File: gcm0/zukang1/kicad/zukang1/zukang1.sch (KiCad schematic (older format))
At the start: 26 parts, among them J1 Conn_01x02_Male, U1 L7805, U2 LM1117-3.3, U3 74HC595, U4 STM32F030F4Px, U5 Si5351A-B-GT, Y1 Crystal, Y2 Crystal_GND24_Small

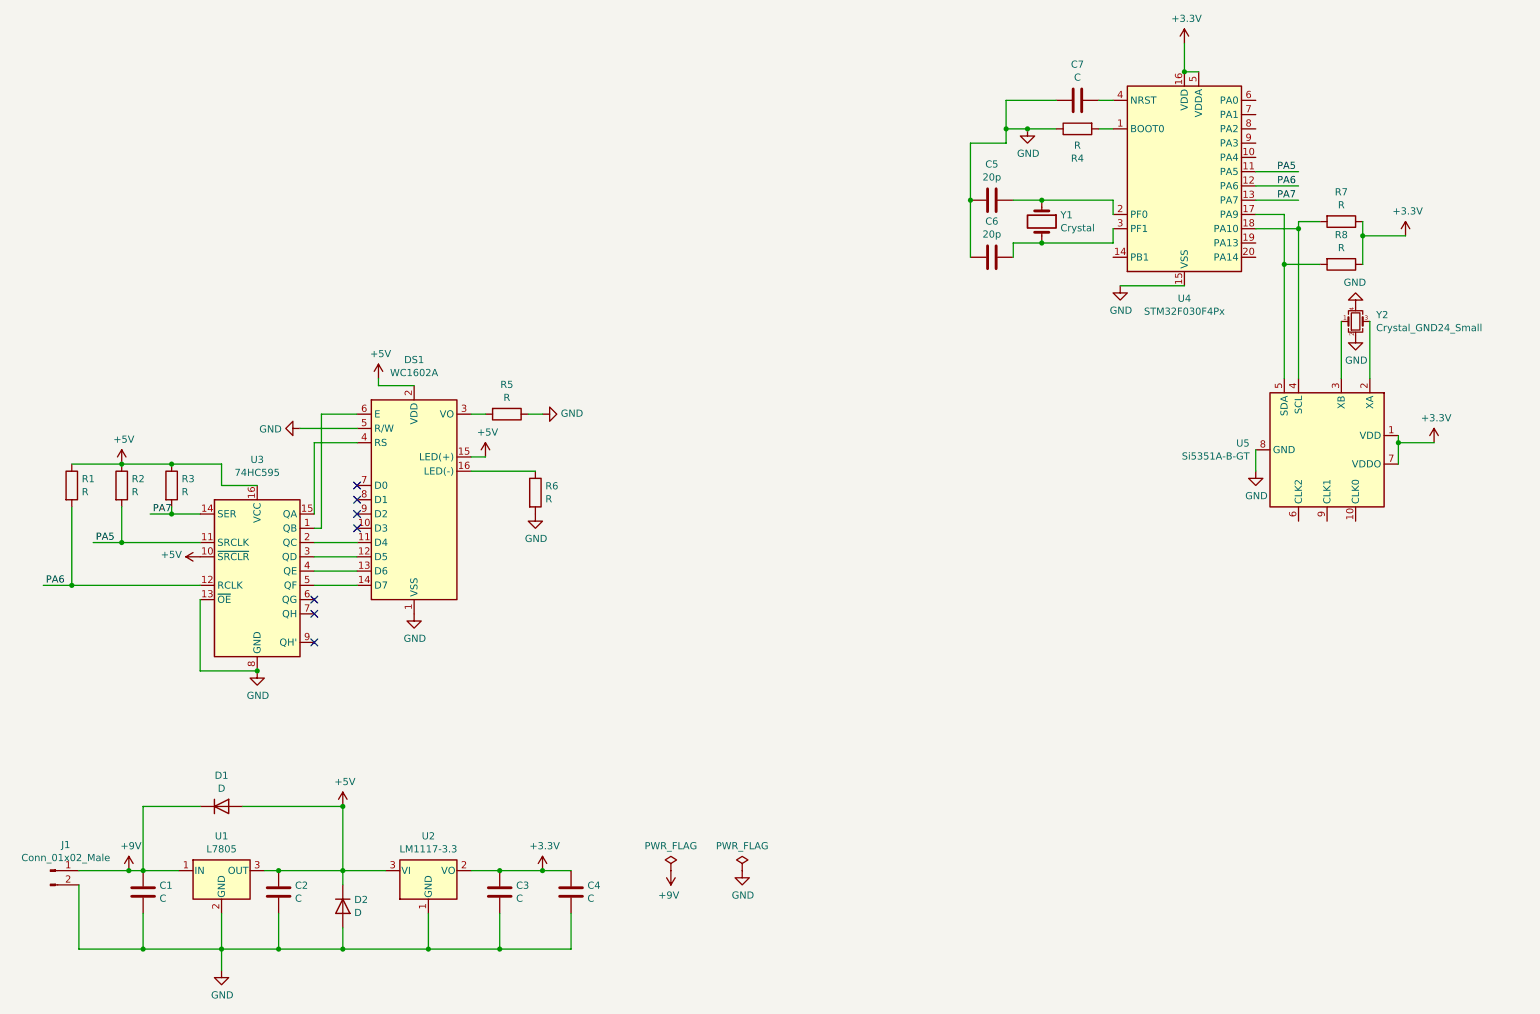
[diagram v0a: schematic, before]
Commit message: 显示PLL
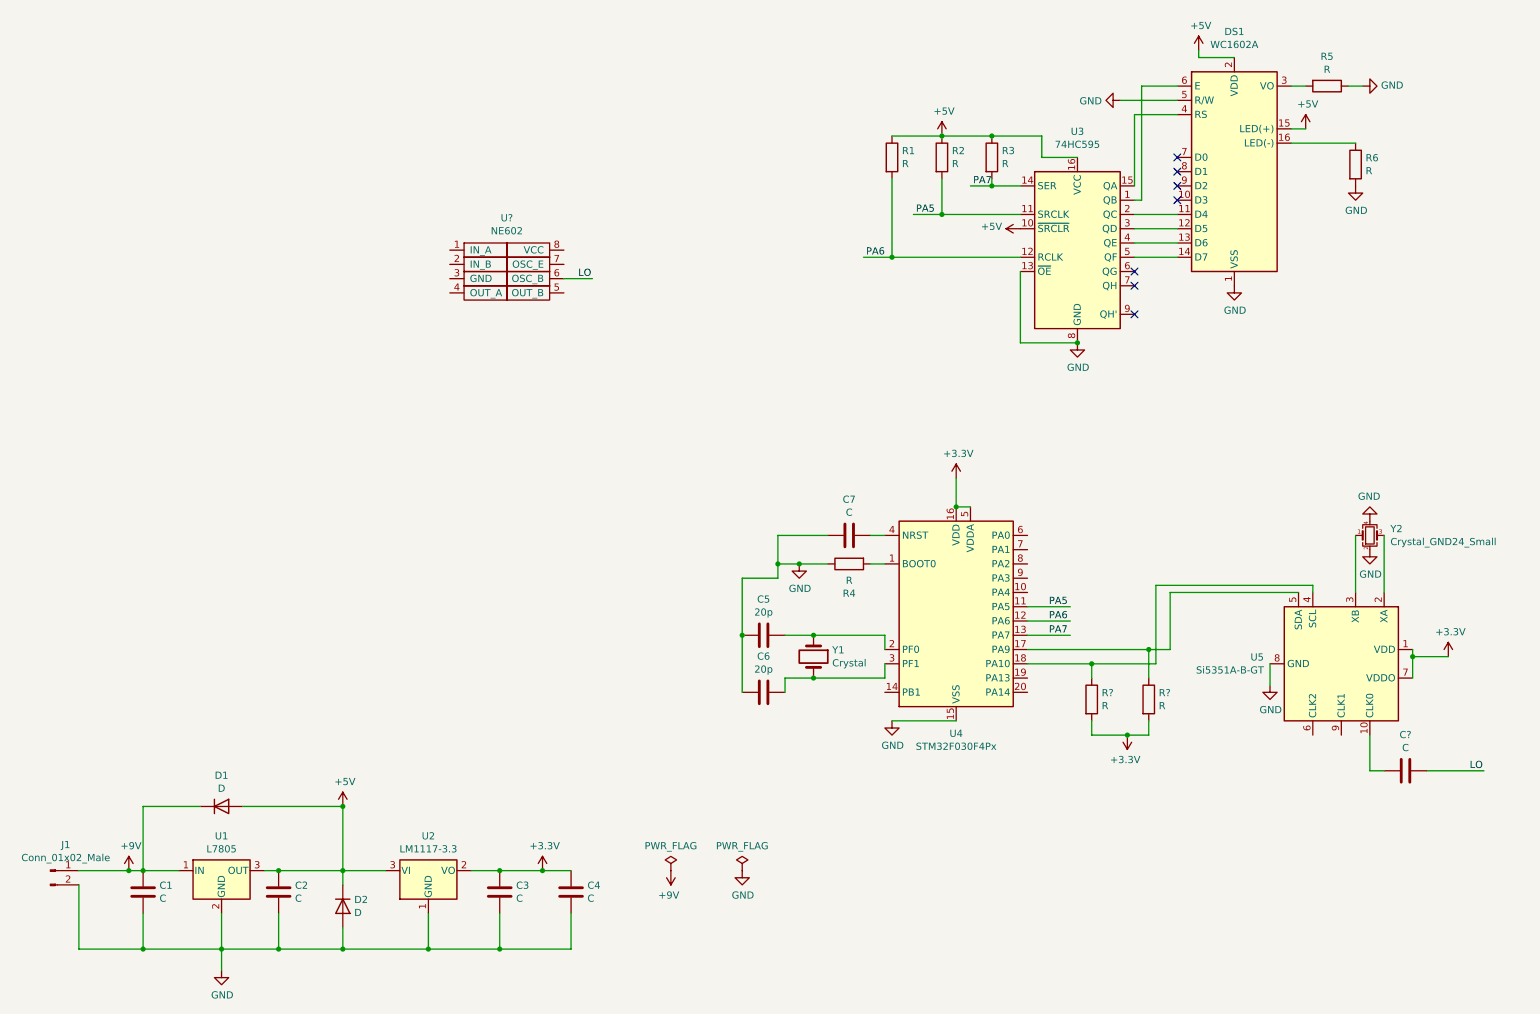
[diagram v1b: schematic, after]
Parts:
- removed R7, R8: R, symbol Device:R
- added C?: C, symbol Device:C
- added R? (x2): R, symbol Device:R
- added U?: NE602, symbol RF:NE602
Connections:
- net labels added: LO
- wire segments 102 -> 110
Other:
- moved on the sheet: C5, C6, C7, DS1, R1, R2, R3, R4, R5, R6, U3, U4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
